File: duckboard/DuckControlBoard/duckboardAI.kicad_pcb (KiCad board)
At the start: 2 copper layers, 154.2 x 127.5 mm, 64 parts, among them J1 BATTERY, J10 Tank Level, J11 5V OUT, J12 PUMP_CONTROL, J14 DOOR_OPEN_LIMIT, J15 DOOR_CLOSE_LIMIT, J16 LIFT_CLOSE_LIMIT, J17PhotoSensor1 Conn_01x02, J2 5V BUCK, J3 LIFT BTS7960, J4 DOOR BTS7960, J6 LIFT CLOSE, J7 LIFT OPEN, J8 DOOR CLOSE, J9 DOOR OPEN, P1 R_Potentiometer, P2 R_Potentiometer, Q1 27P04, Q2 30N06L, U1 ESP32-DevKitC

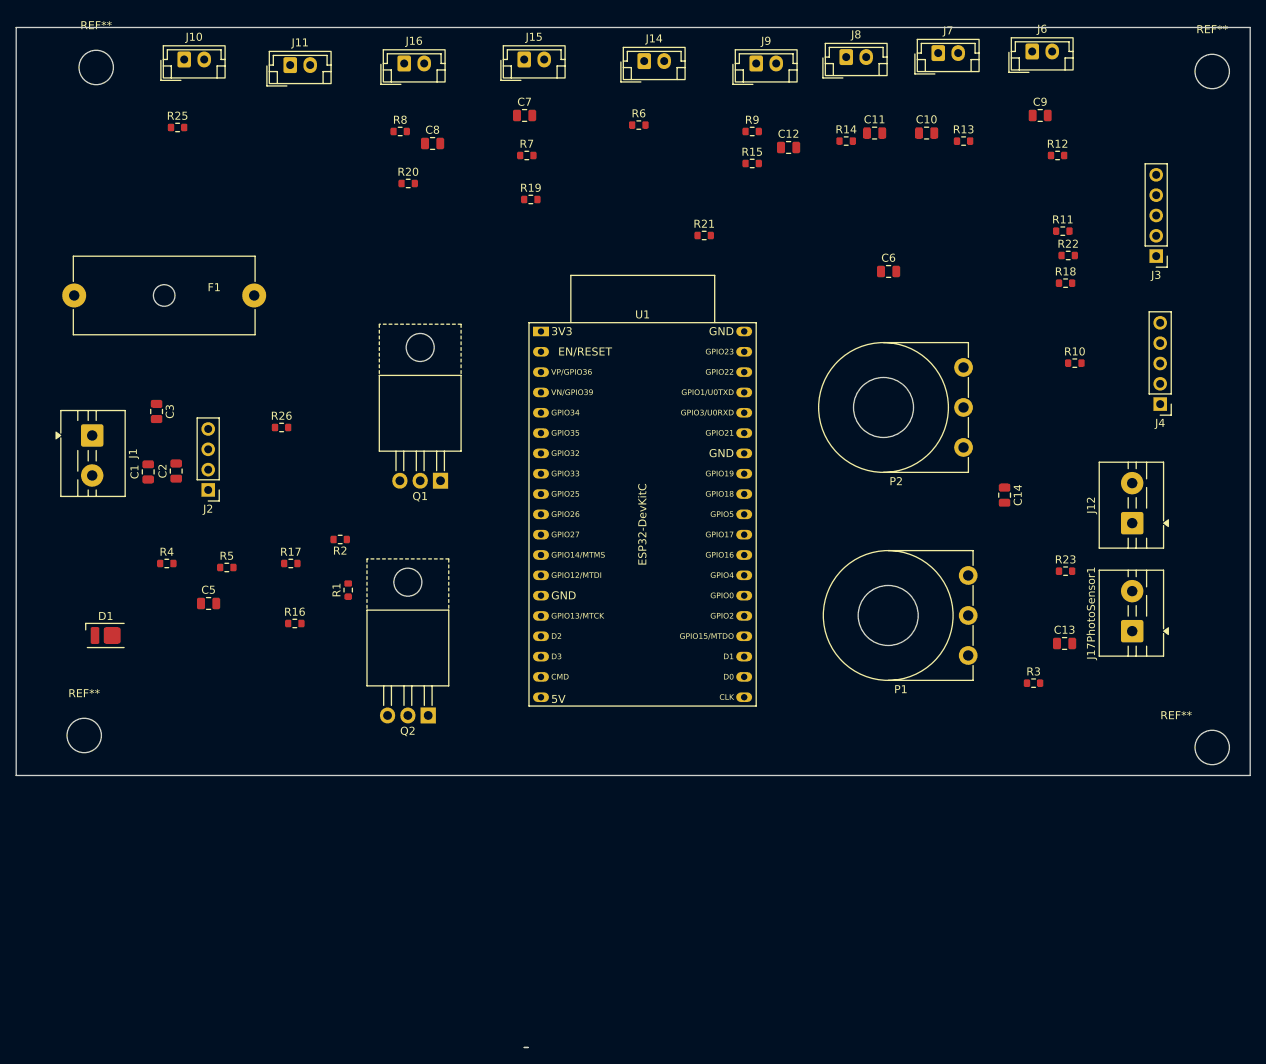
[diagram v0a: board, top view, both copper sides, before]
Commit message: schematic and board work
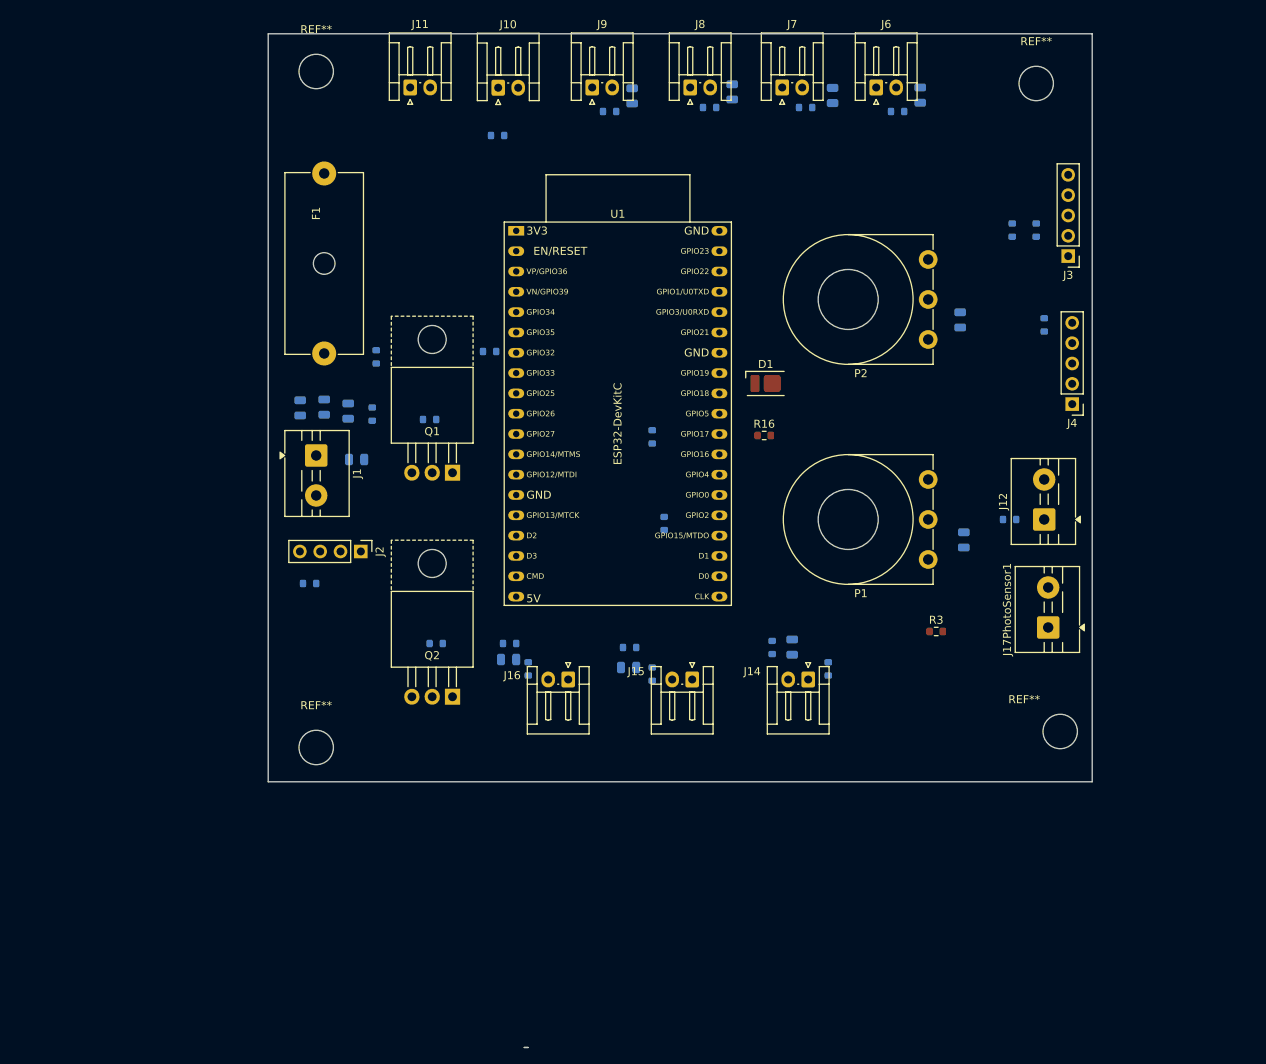
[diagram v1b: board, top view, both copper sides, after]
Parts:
- C1, C10, C11, C12, C13, C14, C2, C3, C5, C6, C7, C8, C9, R1, R10, R11, R12, R13, R14, R15, R17, R18, R19, R2, R20, R21, R22, R23, R25, R26, R4, R5, R6, R7, R8, R9: moved to B.Cu
- J10, J11, J14, J15, J16, J6, J7, J8, J9: footprint Connector_JST:JST_EH_B2B-EH-A_1x02_P2.50mm_Vertical -> Connector_JST:JST_EH_S2B-EH_1x02_P2.50mm_Horizontal
- moved D1 88.3 mm to (177.7, 90.5)
- moved J15 80.3 mm to (168.5, 127.5), turned to 180 degrees
- moved J14 80.0 mm to (183.0, 127.5), turned to 180 degrees
- moved J16 79.7 mm to (153.0, 127.5), turned to 180 degrees
- moved R6 72.0 mm to (185.5, 126.2), turned to 90 degrees
- moved C7 70.2 mm to (160.6, 126.0), turned to 180 degrees
- moved R8 69.1 mm to (148.0, 126.2), turned to -90 degrees
- moved R7 66.7 mm to (163.5, 126.8), turned to -90 degrees
- moved C8 65.2 mm to (145.6, 125.0), turned to 180 degrees
- moved R9 64.5 mm to (178.5, 123.5), turned to -90 degrees
- moved R16 63.2 mm to (177.5, 97.0)
- moved R20 58.9 mm to (145.7, 123.0), turned to 180 degrees
- moved R19 57.3 mm to (160.7, 123.5), turned to 180 degrees
- moved R18 55.1 mm to (163.5, 97.2), turned to -90 degrees
- moved C6 48.5 mm to (181.0, 123.5), turned to -90 degrees
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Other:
- board size 154.2 x 127.5 mm -> 103 x 126.7 mm
